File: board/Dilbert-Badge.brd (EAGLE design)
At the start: 53 x 106.7 mm, 29 parts, among them IC1 MCP23017SO, J1 I2C, J2 UART, J6 IO_B, J7 IO_A, SW1 UP, SW2 DOWN, SW3 LEFT, SW4 RIGHT, SW5 A, SW6 B, SW7 RESET, SW8 SWD

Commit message: More dev work
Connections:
- net N$7 renamed GPIO16
- net TFT_CS renamed GPIO4
- removed net TFT_DC: J5.6, R4.1, X1.11
- net GPIO2: now also J5.6, R4.1, X1.11
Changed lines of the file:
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@@
 <wire x1="41.91" y1="65.77" x2="34.17" y2="64" width="0" layer="19" extent="1-16"/>
 </signal>
-<signal name="N$7">
+<signal name="GPIO16">
 <contactref element="X1" pad="4"/>
 <contactref element="J4" pad="5"/>
@@
 <wire x1="38.1" y1="58.42" x2="34.17" y2="58" width="0" layer="19" extent="1-1"/>
 </signal>
-<signal name="TFT_CS">
+<signal name="GPIO4">
 <contactref element="X1" pad="14"/>
 <contactref element="J5" pad="3"/>
@@
 <signal name="GPIO2">
 <contactref element="R3" pad="1"/>
+<contactref element="J5" pad="6"/>
+<contactref element="X1" pad="11"/>
+<contactref element="R4" pad="1"/>
+<wire x1="19.17" y1="58" x2="15.24" y2="58.42" width="0" layer="19" extent="16-16"/>
+<wire x1="12.7" y1="53.61" x2="15.24" y2="58.42" width="0" layer="19" extent="1-1"/>
+<wire x1="11.43" y1="62.5" x2="15.24" y2="58.42" width="0" layer="19" extent="1-1"/>
 </signal>
 <signal name="N$14">
@@
 <wire x1="5.08" y1="45.45" x2="7.24" y2="28.03" width="0" layer="19" extent="1-1"/>
 </signal>
-<signal name="TFT_DC">
-<contactref element="J5" pad="6"/>
-<contactref element="X1" pad="11"/>
-<contactref element="R4" pad="1"/>
-<wire x1="19.17" y1="58" x2="15.24" y2="58.42" width="0" layer="19" extent="16-16"/>
-<wire x1="12.7" y1="53.61" x2="15.24" y2="58.42" width="0" layer="19" extent="1-1"/>
-</signal>
 </signals>

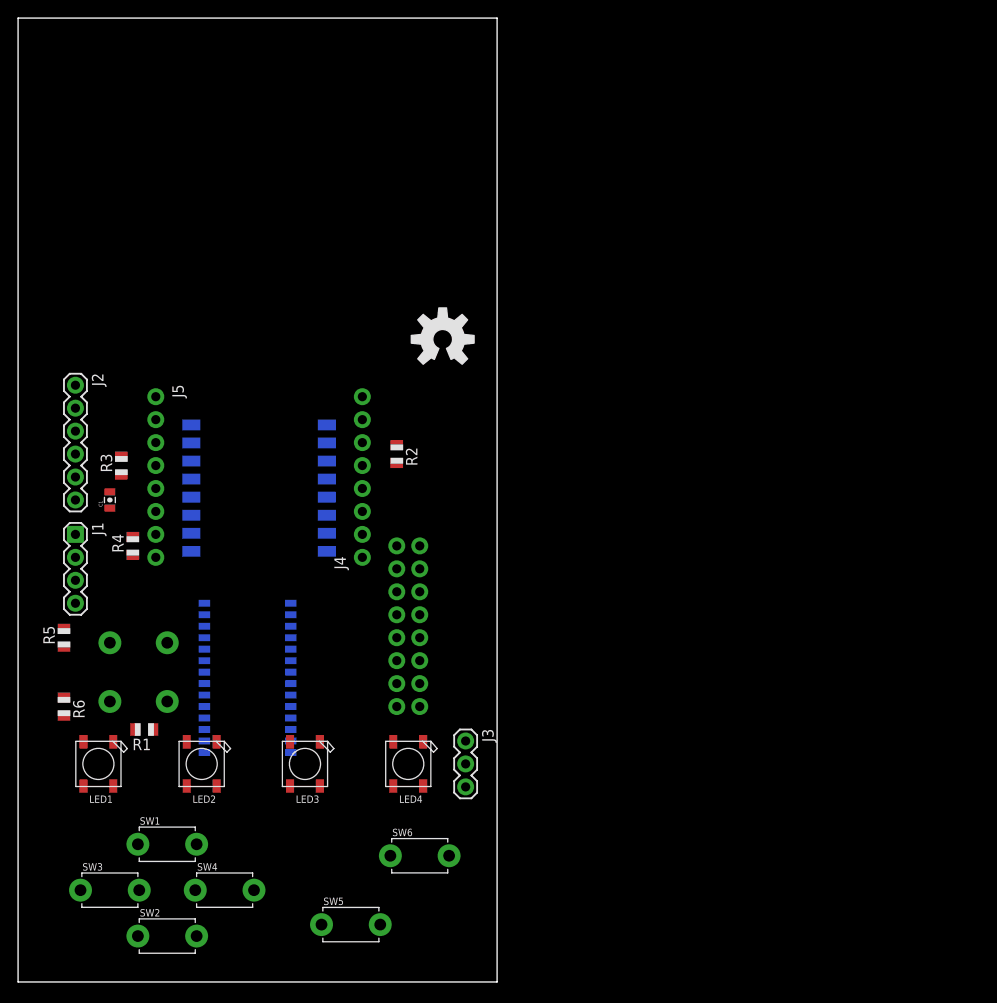
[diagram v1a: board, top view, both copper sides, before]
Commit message: more work on board
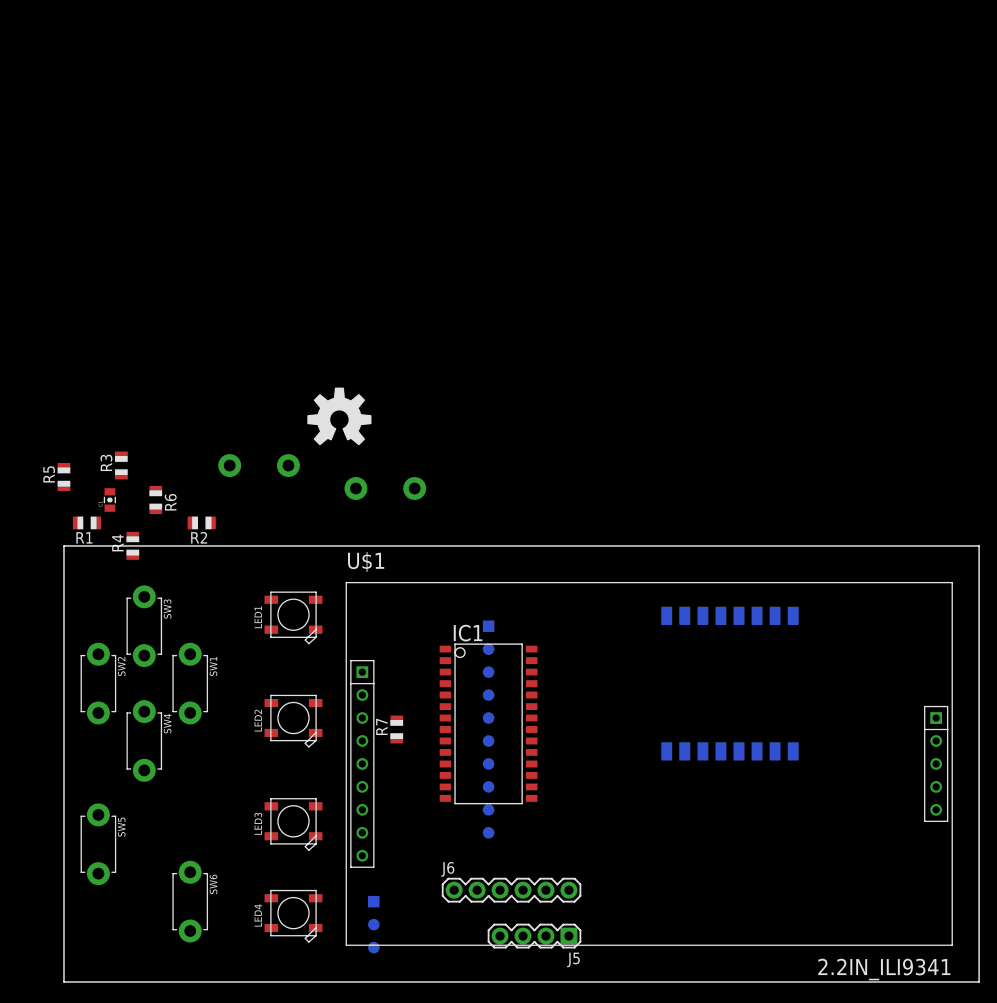
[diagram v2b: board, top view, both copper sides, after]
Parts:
- removed J2: UART, SparkFun-Connectors:1X06
- removed J3: (no value), SparkFun-Connectors:1X03
- removed J4: (no value), SparkFun-Connectors:1X08_NO_SILK
- added R7: 10K, adafruit:R0805
- added U$1: 2.2IN_ILI9341, displays:2.2IN_ILI9341
- J1: value I2C -> (none); device SparkFun-Connectors:1X04 -> connectors:10X1_SMD
- J5: value (none) -> I2C; device SparkFun-Connectors:1X08_NO_SILK -> SparkFun-Connectors:1X04
- J6: value IO_B -> UART; device SparkFun-Connectors:1X08_ROUND -> SparkFun-Connectors:1X06
- J7: value IO_A -> NEOPIXEL; device SparkFun-Connectors:1X08_ROUND -> connectors:3X1_SMD
- moved J5 75.2 mm to (61.0, 11.4), turned to 180 degrees
- moved X1 59.7 mm to (81.3, 39.4), turned to 90 degrees
- moved J1 46.8 mm to (52.1, 45.7), flipped to the bottom
- moved J7 39.7 mm to (39.4, 15.2)
- moved J6 38.6 mm to (48.3, 16.5), flipped to the top, turned to 0 degrees
- moved SW8 36.6 mm to (40.6, 61.0), turned to 180 degrees
- moved SW3 29.5 mm to (14.0, 45.7), turned to 270 degrees
- moved SW5 29.3 mm to (8.89, 21.6), turned to 270 degrees
- moved SW2 29.0 mm to (8.89, 39.4), turned to 270 degrees
- moved LED1 27.2 mm to (30.5, 47.0), turned to 180 degrees
- moved IC1 27.1 mm to (52.1, 35.6), flipped to the top
- moved SW6 25.9 mm to (19.1, 15.2), turned to 270 degrees
- moved R6 25.0 mm to (15.2, 59.7)
- moved SW7 25.0 mm to (26.7, 63.5), turned to 180 degrees
- moved R1 23.7 mm to (7.62, 57.1)
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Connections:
- removed net N$14: IC1.1, J6.1
- removed net N$15: IC1.2, J6.2
- removed net N$16: IC1.8, J6.8
- removed net N$17: IC1.7, J6.7
- removed net N$18: IC1.6, J6.6
- removed net N$19: IC1.5, J6.5
- removed net N$20: IC1.4, J6.4
- removed net N$21: IC1.3, J6.3
- removed net N$22: IC1.28, J7.8
- removed net N$23: IC1.27, J7.7
- new net N$10: IC1.8, J1.8
- new net N$11: IC1.7, J1.7
- new net N$12: IC1.6, J1.6
- new net N$13: IC1.5, J1.5
- new net N$4: IC1.1, J1.1
- new net N$5: IC1.2, J1.2
- new net N$6: IC1.3, J1.3
- new net N$7: IC1.4, J1.4
- new net N$8: IC1.28, J1.10
- new net N$9: IC1.27, J1.9
- new net SD_CS: U$1.SD_CS
- new net TFT_BL: U$1.LED
- new net TFT_CS: U$1.CS
- new net TFT_DC: U$1.DC
- new net TFT_RESET: R7.1, U$1.RESET
- net 3V3: now also J5.2, J6.4, J7.2, R7.2, U$1.VCC; no longer J1.2, J2.4, J3.2, J4.1
- net BTN_A: no longer J7.5
- net BTN_B: no longer J7.6
- net BTN_D: no longer J7.2
- net BTN_L: no longer J7.3
- net BTN_R: no longer J7.4
- net BTN_U: no longer J7.1
- net ESP_ADC: no longer J4.7
- net ESP_CH_PD: no longer J4.6
- net GND: now also J5.1, J6.6, J7.1, U$1.GND; no longer J1.1, J2.6, J3.1, J5.8
- net GPIO16: no longer J4.5
- net GPIO2: no longer J5.6
- net GPIO4: no longer J5.3
- net MISO: now also U$1.MISO, U$1.SD_MISO; no longer J4.3
- net MOSI: now also U$1.MOSI, U$1.SD_MOSI; no longer J4.2
- net NEOPIXEL: no longer J5.7
- net NEOPIXEL_OUT: now also J7.3; no longer J3.3
- net RESET: no longer J4.8
- net SCK: now also U$1.SCK, U$1.SD_SCK; no longer J4.4
- net SCL: now also J5.4; no longer J1.4, J5.5
- net SDA: now also J5.3; no longer J1.3, J5.4
- net UART_CTS: now also J6.5; no longer J2.5
- net UART_DTR: now also J6.1; no longer J2.1
- net UART_RX: now also J6.3; no longer J2.3, J5.2
- net UART_TX: now also J6.2; no longer J2.2, J5.1
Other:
- board size 53 x 106.7 mm -> 101.3 x 48.2 mm

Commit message: more work
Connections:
- removed net GPIO16: X1.4
- removed net GPIO4: X1.14
- new net GPIO0: R5.1, SW8.P$2, X1.12
- net SCL: now also X1.13; no longer R5.1, SW8.P$2, X1.12
- net SDA: now also X1.14; no longer X1.13
- net TFT_BL: now also X1.4
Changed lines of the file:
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@@
 </signal>
 <signal name="SDA">
-<contactref element="X1" pad="13"/>
 <contactref element="IC1" pad="13"/>
 <contactref element="J5" pad="3"/>
-<wire x1="47.29" y1="27.94" x2="79.78" y2="46.87" width="0" layer="19" extent="1-16"/>
+<contactref element="X1" pad="14"/>
+<wire x1="47.29" y1="27.94" x2="81.78" y2="46.87" width="0" layer="19" extent="1-16"/>
 <wire x1="55.88" y1="11.43" x2="47.29" y2="27.94" width="0" layer="19" extent="1-1"/>
 </signal>
 <signal name="SCL">
-<contactref element="X1" pad="12"/>
 <contactref element="IC1" pad="12"/>
-<contactref element="SW8" pad="P$2"/>
-<contactref element="R5" pad="1"/>
 <contactref element="J5" pad="4"/>
-<wire x1="47.29" y1="29.21" x2="77.78" y2="46.87" width="0" layer="19" extent="1-16"/>
+<contactref element="X1" pad="13"/>
+<wire x1="47.29" y1="29.21" x2="79.78" y2="46.87" width="0" layer="19" extent="1-16"/>
 <wire x1="53.34" y1="11.43" x2="47.29" y2="29.21" width="0" layer="19" extent="1-1"/>
-<wire x1="43.89" y1="60.96" x2="47.29" y2="29.21" width="0" layer="19" extent="1-1"/>
-<wire x1="5.08" y1="61.23" x2="43.89" y2="60.96" width="0" layer="19" extent="1-1"/>
 </signal>
 <signal name="UART_TX">
@@
 <wire x1="21.32" y1="57.15" x2="81.78" y2="31.87" width="0" layer="19" extent="1-16"/>
 </signal>
-<signal name="GPIO16">
-<contactref element="X1" pad="4"/>
-</signal>
 <signal name="SCK">
 <contactref element="X1" pad="5"/>
@@
 <wire x1="75.78" y1="31.87" x2="101.6" y2="30.48" width="0" layer="19" extent="16-16"/>
 <wire x1="38.1" y1="20.32" x2="75.78" y2="31.87" width="0" layer="19" extent="16-16"/>
-</signal>
-<signal name="GPIO4">
-<contactref element="X1" pad="14"/>
 </signal>
 <signal name="GPIO2">
@@
 <signal name="TFT_BL">
 <contactref element="U$1" pad="LED"/>
+<contactref element="X1" pad="4"/>
+<wire x1="38.1" y1="22.86" x2="79.78" y2="31.87" width="0" layer="19" extent="16-16"/>
 </signal>
 <signal name="TFT_DC">
@@
 <wire x1="52.07" y1="35.56" x2="47.29" y2="38.1" width="0" layer="19" extent="1-1"/>
 </signal>
+<signal name="GPIO0">
+<contactref element="X1" pad="12"/>
+<contactref element="SW8" pad="P$2"/>
+<contactref element="R5" pad="1"/>
+<wire x1="43.89" y1="60.96" x2="77.78" y2="46.87" width="0" layer="19" extent="16-16"/>
+<wire x1="5.08" y1="61.23" x2="43.89" y2="60.96" width="0" layer="19" extent="1-1"/>
+</signal>
 </signals>
